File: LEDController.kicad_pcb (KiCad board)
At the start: 2 copper layers, 18 parts, among them J1 3557-2, J11 TB002-500-04BE, J12 TB002-500-04BE, J16 3557-2, J17 TB002-500-04BE, J2 3557-2, J3 3557-2, J4 3557-2, J5 3557-2, J6 3557-2, J7 0389690002, J8 3557-2, J9 Conn_01x03_Pin, K1 J115F11CH5VDCS61.5U, Q1 BCX56,135

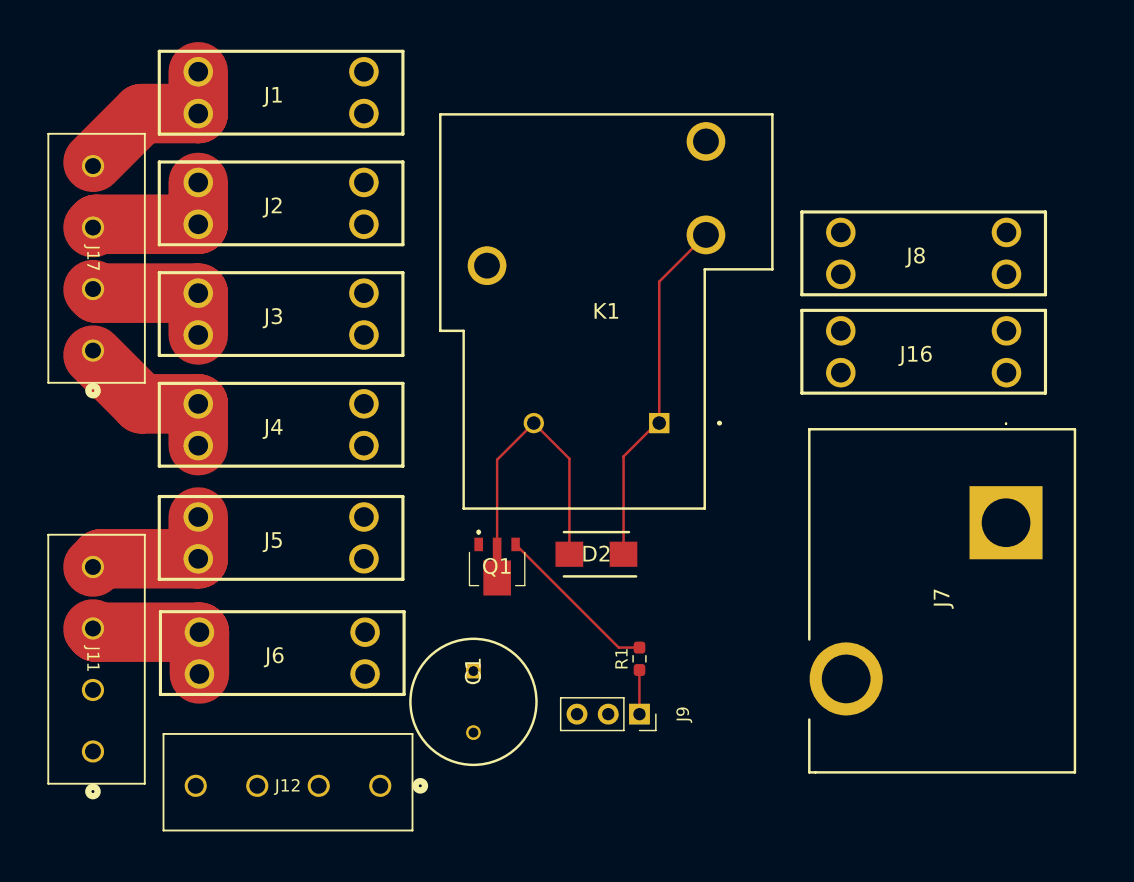
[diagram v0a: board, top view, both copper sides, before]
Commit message: wip layout
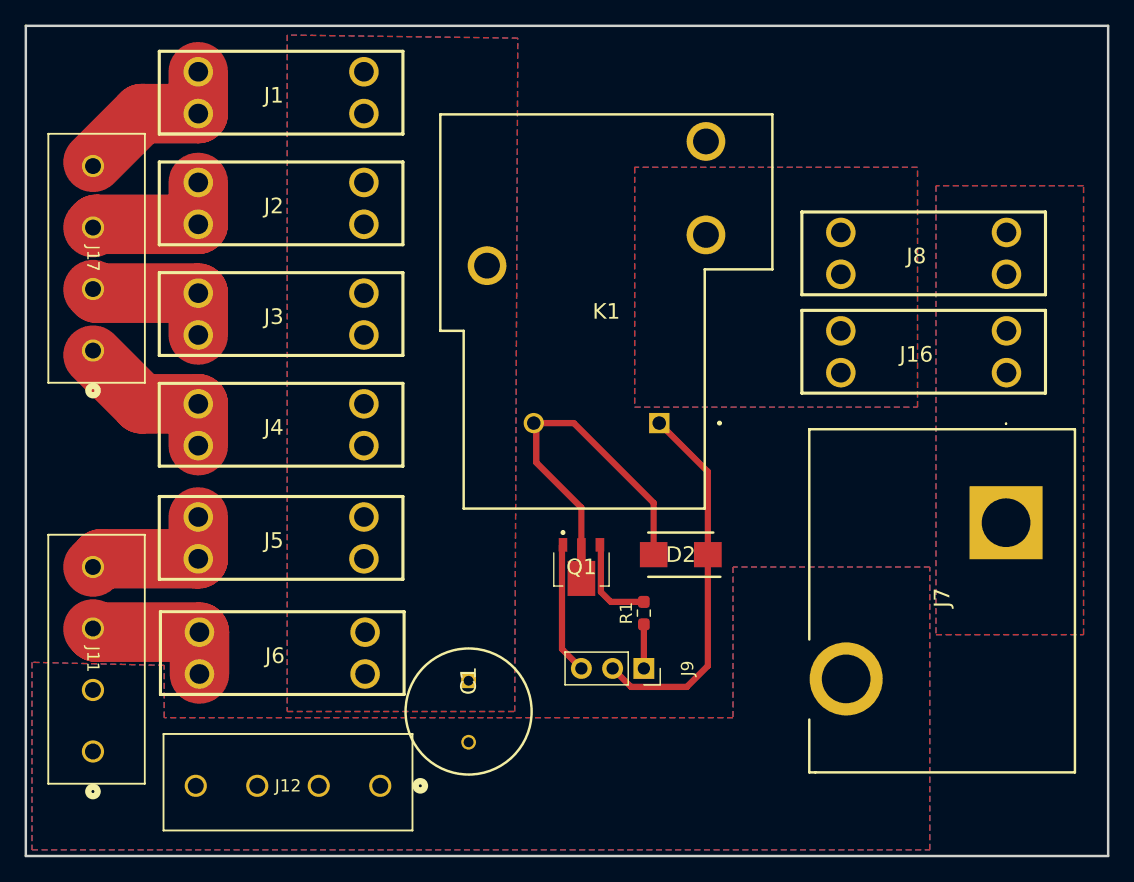
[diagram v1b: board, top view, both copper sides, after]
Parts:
- C1: footprint SamacSys_Parts:CAPPRD500W60D1025H2200 -> LEDController:CAPPRD500W60D1025H2200
- D2: footprint SamacSys_Parts:DIOM5336X240N -> LEDController:DIOM5336X240N
- J1, J16, J2, J3, J4, J5, J6, J8: footprint SamacSys_Parts:3557-2 -> LEDController:3557-2
- J11, J12, J17: footprint SamacSys_Parts:CONN4_TB002-500_787x299_CUD -> LEDController:CONN4_TB002-500_787x299_CUD
- J7: footprint SamacSys_Parts:0389690002 -> LEDController:0389690002
- K1: footprint SamacSys_Parts:J115F11CH5VDCS615U -> LEDController:J115F11CH5VDCS615U
- Q1: footprint SamacSys_Parts:PBSS4360XX -> LEDController:PBSS4360XX
- moved D2 6.86 mm to (98.5, 104.6)
- moved Q1 6.86 mm to (90.4, 105.6)
- moved J9 3.73 mm to (95.5, 113.8)
- moved R1 3.73 mm to (95.5, 109.3)
- moved C1 0.88 mm to (81.2, 114.8)
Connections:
- D2 pad 1: Net-(D2-K) -> /50F
- D2 pad 2: Net-(C1-+) -> Net-(D2-A)
- K1 pad 1: Net-(D2-K) -> /50F
- K1 pad 2: Net-(C1-+) -> Net-(D2-A)
- K1 pad 3: Net-(C1-+) -> /50R
- K1 pad 5: Net-(D2-K) -> /50F
- Q1 pad 2: Net-(C1-+) -> Net-(D2-A)
- Q1 pad 4: Net-(C1-+) -> Net-(D2-A)
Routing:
- net /50F: track 0.00 -> 30.5 mm
- net Net-(D2-K): track 29.1 -> 0.00 mm
- net Net-(D2-A): track 0.00 -> 28.5 mm
- net Net-(C1-+): track 23.3 -> 0.00 mm
- net GND: track 0.00 -> 10.7 mm
- net Net-(Q1-B): track 13.5 -> 7.69 mm
- added copper zone on B.Cu, net /50F
- added copper zone on F.Cu, net /50F
- added copper zone on B.Cu, net /50R
- added copper zone on F.Cu, net /50R
- added copper zone on B.Cu, net /50U
- added copper zone on F.Cu, net /50U
- added copper zone on B.Cu, net GND
- added copper zone on F.Cu, net GND
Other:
- board outline added: 88 x 67.5 mm
